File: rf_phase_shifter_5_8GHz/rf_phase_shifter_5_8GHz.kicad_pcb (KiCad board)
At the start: 2 copper layers, 12 parts, among them J1 CON-SMA-EDGE-S, J2 CON-SMA-EDGE-S, J3 CON-SMA-EDGE-S

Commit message: pcb init works
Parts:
- L1, L2: value 1u -> 220n

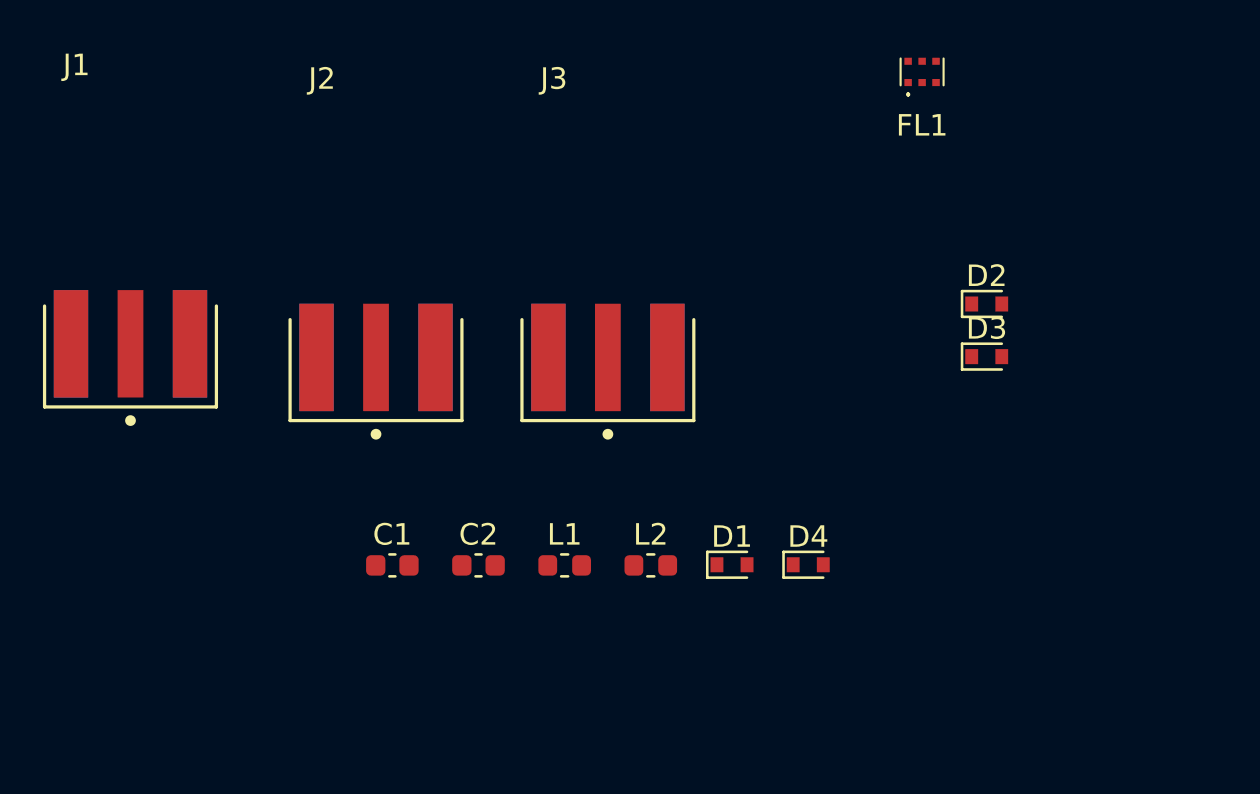
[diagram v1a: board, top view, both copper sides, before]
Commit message: finished pcb layouts
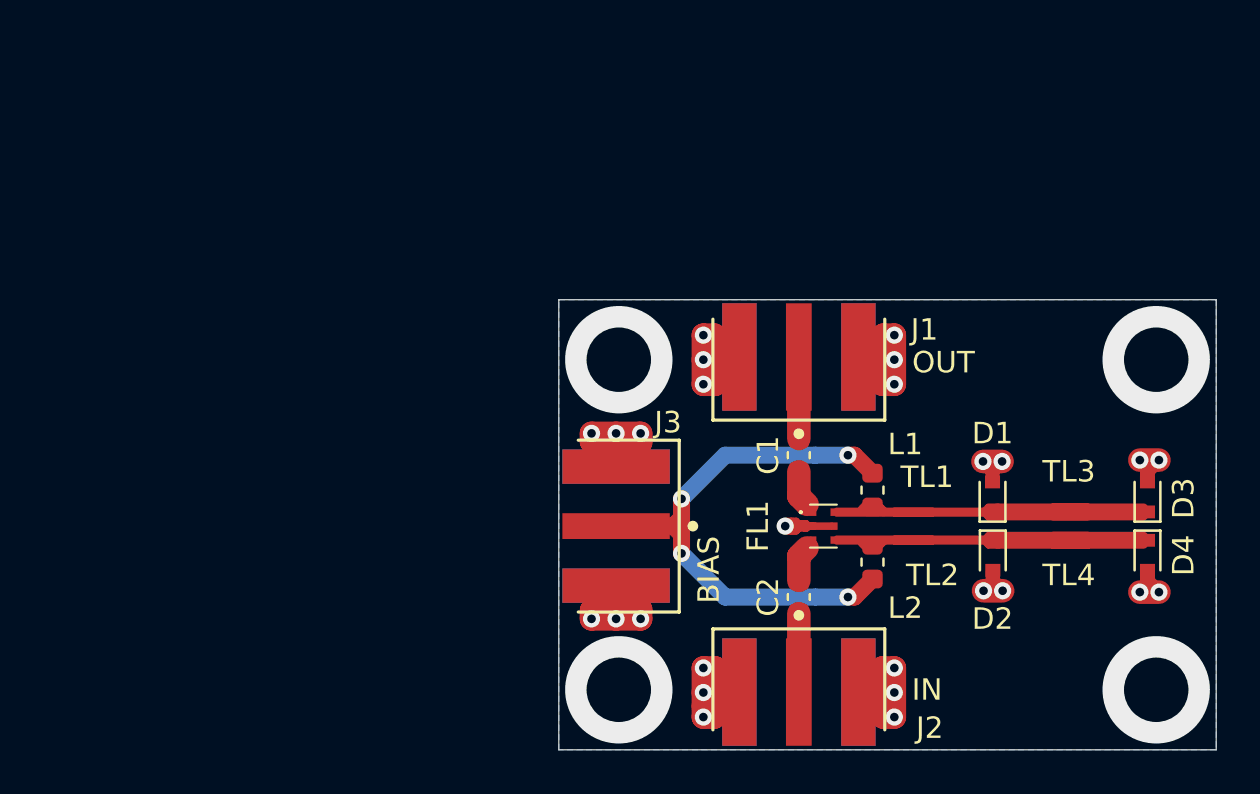
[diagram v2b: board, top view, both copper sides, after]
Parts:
- added TL1: TL_13_5_8GHz, analog_rf_phase_shifter_module:TL_13_5_8GHz, F.Cu at (89.8, 58.3)
- added TL2: TL_13_5_8GHz, analog_rf_phase_shifter_module:TL_13_5_8GHz, F.Cu at (89.8, 59.6)
- added TL3: TL_24_5_8GHz, analog_rf_phase_shifter_module:TL_24_5_8GHz, F.Cu at (97.1, 58.3)
- added TL4: TL_24_5_8GHz, analog_rf_phase_shifter_module:TL_24_5_8GHz, F.Cu at (97.1, 59.6)
- moved J2 36.0 mm to (84.5, 73.9), turned to 180 degrees
- moved J1 31.1 mm to (84.5, 43.8)
- moved FL1 21.6 mm to (85.6, 58.9), turned to 270 degrees
- moved C1 19.6 mm to (84.5, 55.6), turned to 90 degrees
- moved J3 16.6 mm to (68.7, 58.9), turned to 90 degrees
- moved D4 15.8 mm to (100.7, 60.3), turned to 270 degrees
- moved C2 15.0 mm to (84.5, 62.2), turned to 90 degrees
- moved L1 14.8 mm to (87.9, 57.3), turned to 270 degrees
- moved D1 12.5 mm to (93.5, 57.6), turned to 90 degrees
- moved D2 11.7 mm to (93.5, 60.3), turned to 270 degrees
- moved L2 10.3 mm to (87.9, 60.6), turned to 90 degrees
- moved D3 9.93 mm to (100.7, 57.6), turned to 90 degrees
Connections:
- D3 pad 1: Net-(D1-Pad1) -> Net-(D3-Pad1)
- D4 pad 1: Net-(D2-Pad1) -> Net-(D4-Pad1)
- FL1 pad 4: Net-(D2-Pad1) -> Net-(FL1-Pad4)
- FL1 pad 6: Net-(D1-Pad1) -> Net-(FL1-Pad6)
- L1 pad 2: Net-(D1-Pad1) -> Net-(FL1-Pad6)
- L2 pad 2: Net-(D2-Pad1) -> Net-(FL1-Pad4)
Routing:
- net GND: track 0.00 -> 69.4 mm, vias 0 -> 31
- net Net-(J3-Pad1): track 0.00 -> 28.3 mm, vias 0 -> 4
- net Net-(D2-Pad1): track 0.00 -> 9.90 mm
- net Net-(D1-Pad1): track 0.00 -> 6.29 mm
- net Net-(C1-Pad2): track 0.00 -> 3.65 mm
- net Net-(C2-Pad1): track 0.00 -> 3.65 mm
- net Net-(C2-Pad2): track 0.00 -> 1.67 mm
- net Net-(C1-Pad1): track 0.00 -> 1.67 mm
- net Net-(FL1-Pad4): track 0.00 -> 1.17 mm
- net Net-(FL1-Pad6): track 0.00 -> 0.90 mm
- added copper zone on B.Cu, net GND
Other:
- board outline added: 30.6 x 21 mm
- board text added: "Analog RF phase shifter 5.8GHz Marcin Wachowiak, Poland"
- board text added: "BIAS"
- board text added: "IN"
- board text added: "OUT"
